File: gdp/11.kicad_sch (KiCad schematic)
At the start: 5 parts, among them IC15 74LS367, IC26 74LS374, IC27 74LS374, IC33 74LS244, IC34 74LS244

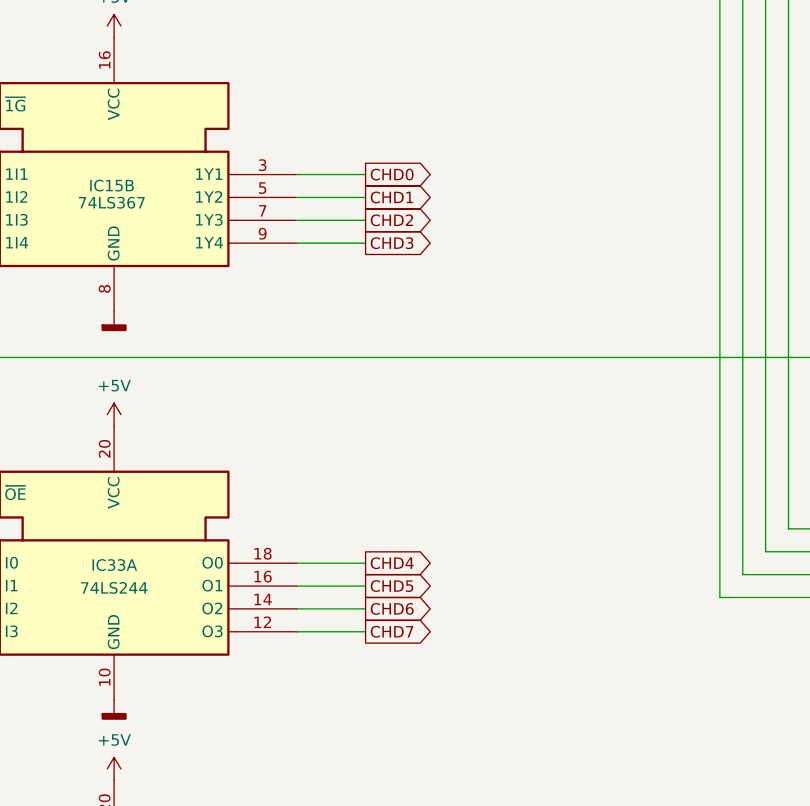
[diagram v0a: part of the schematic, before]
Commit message: Bug fix
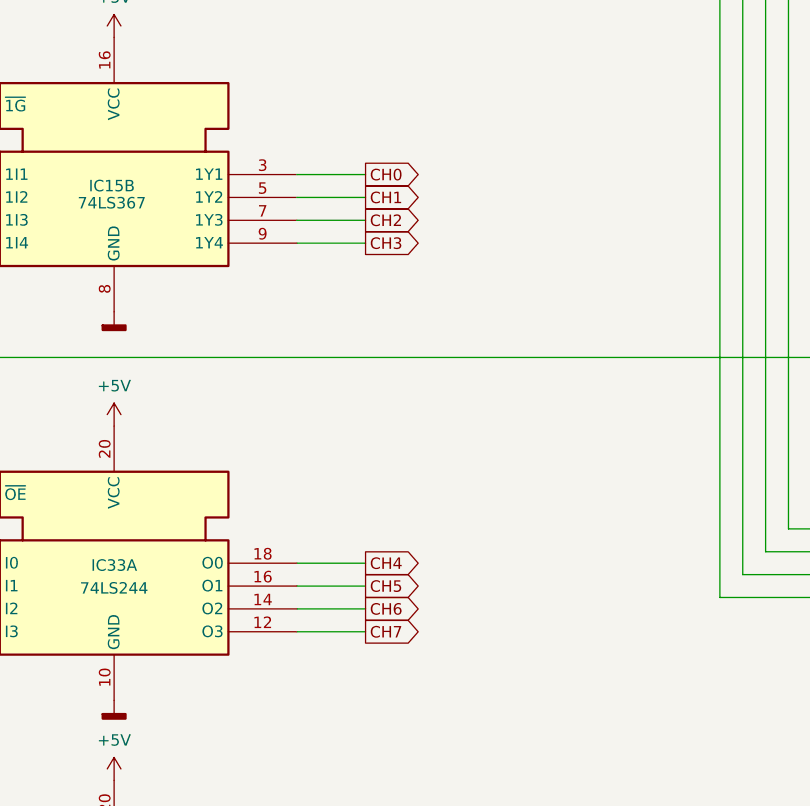
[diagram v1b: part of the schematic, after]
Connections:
- net CH0: now also IC15.3 (1Y1)
- net CH1: now also IC15.5 (1Y2)
- net CH2: now also IC15.7 (1Y3)
- net CH3: now also IC15.9 (1Y4)
- net CH4: now also IC33.18 (O0)
- net CH5: now also IC33.16 (O1)
- net CH6: now also IC33.14 (O2)
- net CH7: now also IC33.12 (O3)
- net CHD0: no longer IC15.3 (1Y1)
- net CHD1: no longer IC15.5 (1Y2)
- net CHD2: no longer IC15.7 (1Y3)
- net CHD3: no longer IC15.9 (1Y4)
- net CHD4: no longer IC33.18 (O0)
- net CHD5: no longer IC33.16 (O1)
- net CHD6: no longer IC33.14 (O2)
- net CHD7: no longer IC33.12 (O3)
